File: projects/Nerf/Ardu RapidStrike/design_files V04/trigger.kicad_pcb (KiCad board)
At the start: 2 copper layers, 35 x 33 mm, 19 parts, among them J19 TRIG, J20 PUSH, J21 BUTTON, J22 TRIG_OUT, J6 REV, U7 74LS14

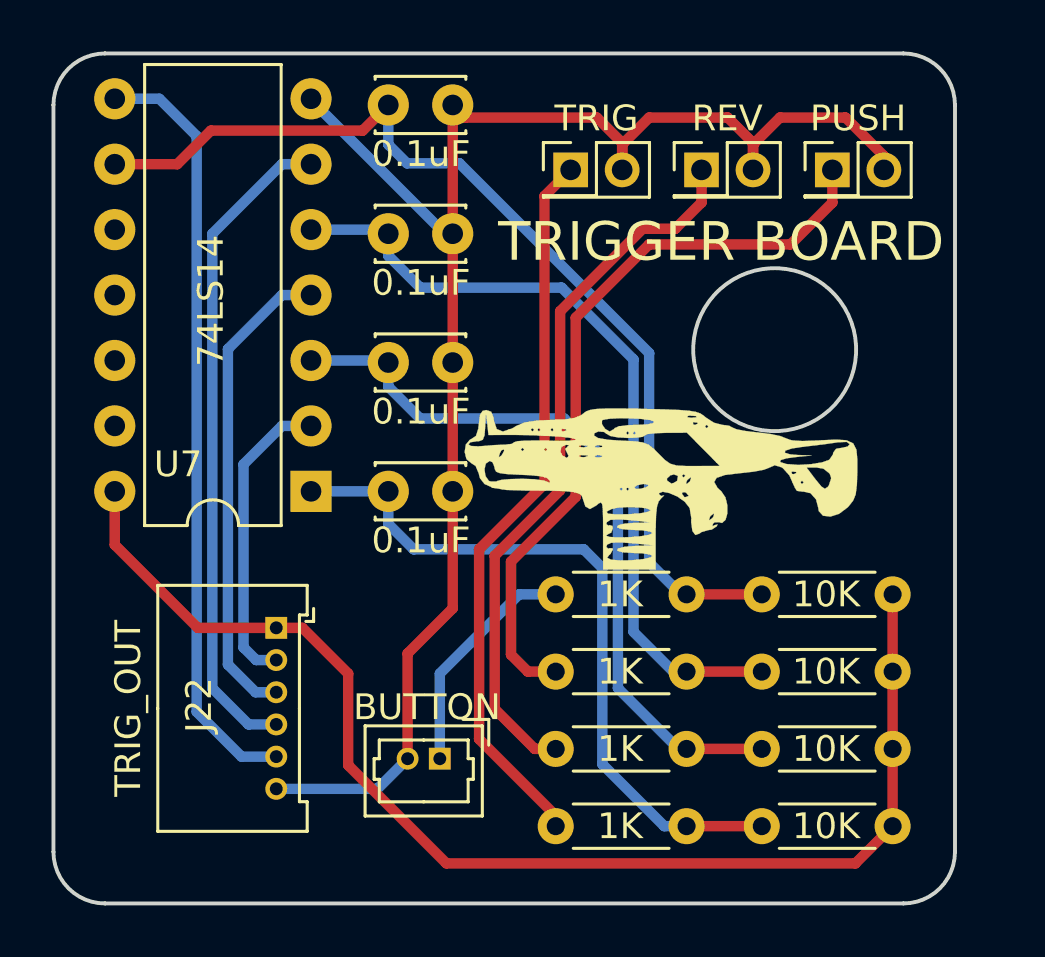
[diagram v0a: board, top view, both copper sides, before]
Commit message: Updates
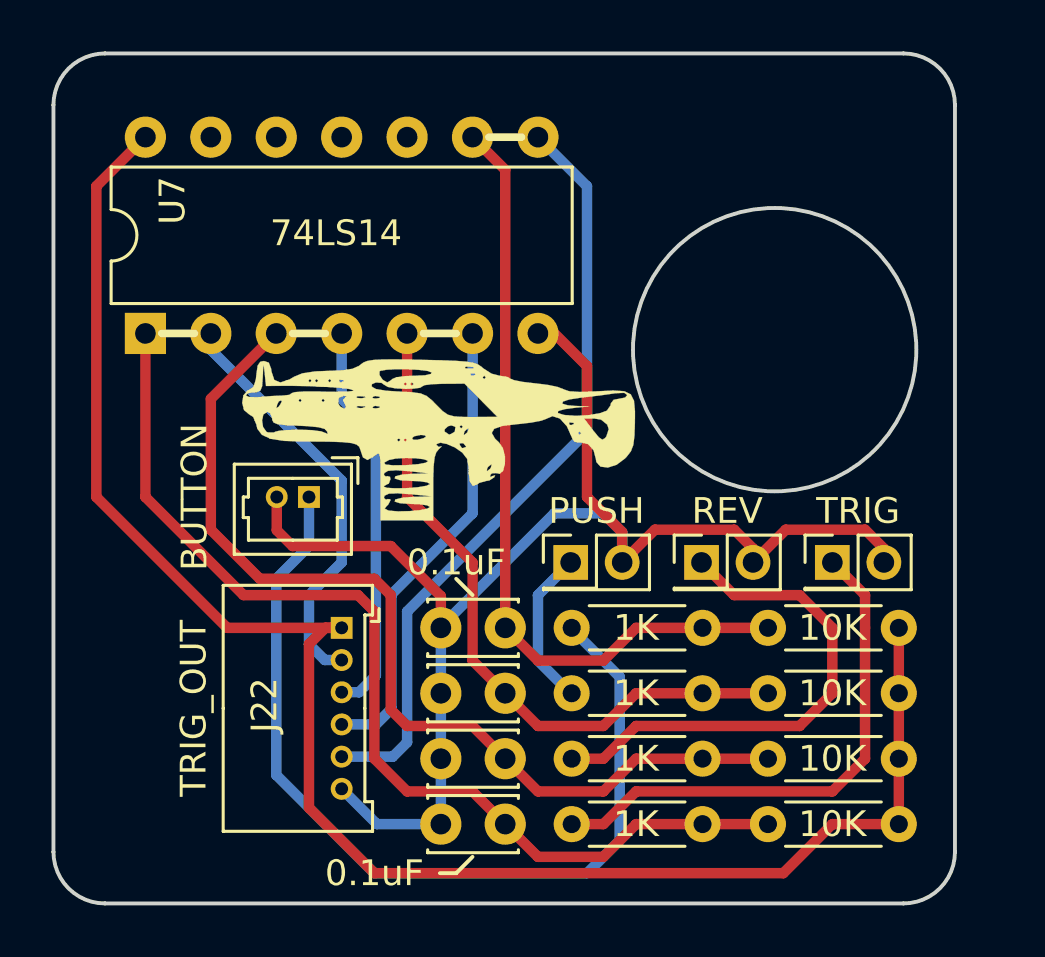
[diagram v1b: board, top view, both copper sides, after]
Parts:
- moved C10 20.8 mm to (240.5, 113.7), turned to 180 degrees
- moved C8 18.4 mm to (240.5, 116.2), turned to 180 degrees
- moved J19 18.3 mm to (253.2, 111.1)
- moved J20 18.3 mm to (243.1, 111.1)
- moved C7 16.0 mm to (240.5, 118.7), turned to 180 degrees
- moved J6 15.2 mm to (248.2, 111.1)
- moved C6 13.7 mm to (240.5, 121.3), turned to 180 degrees
- moved J21 11.4 mm to (232.9, 108.6)
- moved U7 8.88 mm to (226.6, 102.2), turned to 90 degrees
- moved G*** 8.84 mm to (238.0, 105.4)
- moved J22 2.54 mm to (234.2, 113.7)
- moved R18 1.44 mm to (245.6, 113.7)
- moved R19 1.32 mm to (253.2, 113.7)
- moved R11 1.04 mm to (245.6, 116.2)
- moved R10 0.87 mm to (253.2, 116.2)
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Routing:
- net Net-(J21-Pad1): track 9.08 -> 35.8 mm
- net Net-(J20-Pad1): track 29.7 -> 6.17 mm
- net VCC: track 49.2 -> 66.8 mm
- net Net-(C6-Pad1): track 28.1 -> 40.9 mm
- net Net-(C10-Pad1): track 39.6 -> 30.9 mm
- net Net-(J6-Pad1): track 28.0 -> 19.8 mm
- net Net-(C7-Pad1): track 29.6 -> 37.7 mm
- net Net-(J19-Pad1): track 28.2 -> 20.6 mm
- net /PUSHER: track 25.7 -> 18.1 mm
- net GND: track 63.3 -> 55.9 mm
- net Net-(C8-Pad1): track 31.5 -> 26.8 mm
- net /TRIG: track 11.8 -> 16.2 mm
- net /REV: track 19.0 -> 15.4 mm
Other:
- outline, holes or cut-outs redrawn
- board text added: "Todo: Fit check pusher board"
